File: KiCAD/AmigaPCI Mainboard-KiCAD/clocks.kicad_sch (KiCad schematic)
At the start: 30 parts, among them CN201 I2C, U108 74AHCT04, U201 Si5351A-B-GM, U210 AT27C4096, U211 AT27C4096, U219 74HCT04, U906 AT27C1024, U907 AT27C1024, Y3 25MHz

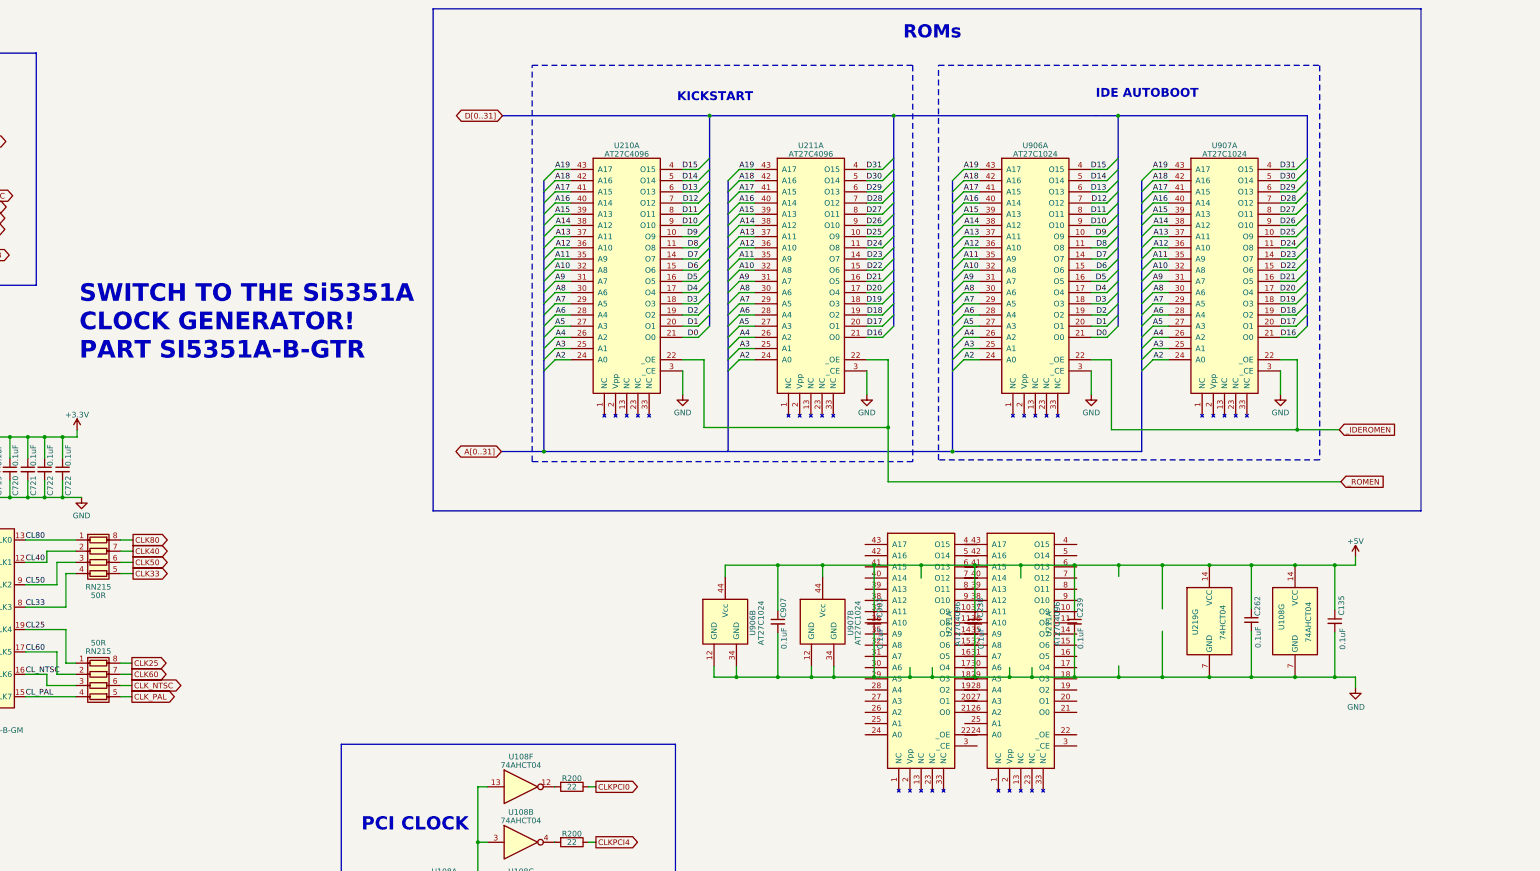
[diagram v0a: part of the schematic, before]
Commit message: Schematic and Routing 14-DEC-2023
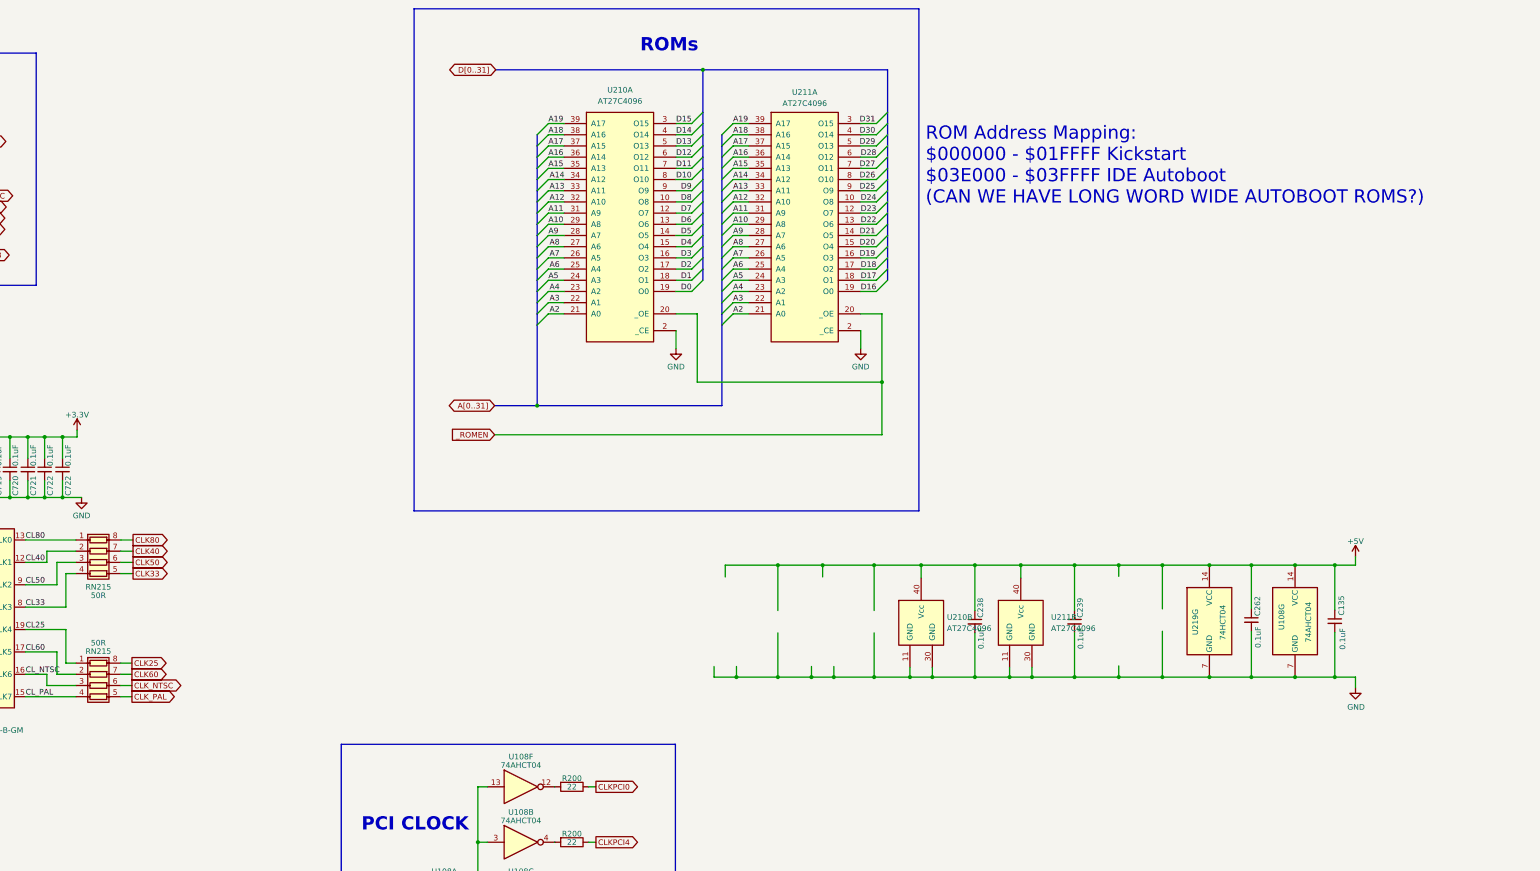
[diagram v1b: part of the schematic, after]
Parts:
- removed C903, C907: 0.1uF, Capacitor_SMD:C_0603_1608Metric, symbol Device:C_Small
- removed U210, U211 (x3): AT27C4096, Package_LCC:PLCC-44_SMD-Socket, symbol AmigaPCI-Symbols:AT27C4096-PLCC
- removed U906, U907: AT27C1024, Package_LCC:PLCC-44_SMD-Socket, symbol AmigaPCI-Symbols:AT27C4096-PLCC
- added U210, U211: AT27C4096, Package_DIP:DIP-40_W16.51mm_SMDSocket_LongPads, symbol AmigaPCI-Symbols:AT27C4096
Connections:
- net +5V: now also U210.40 (Vcc), U211.40 (Vcc)
- net A10: now also U210.29 (A8), U211.29 (A8)
- net A11: now also U210.31 (A9), U211.31 (A9)
- net A12: now also U210.32 (A10), U211.32 (A10)
- net A13: now also U210.33 (A11), U211.33 (A11)
- net A14: now also U210.34 (A12), U211.34 (A12)
- net A15: now also U210.35 (A13), U211.35 (A13)
- net A16: now also U210.36 (A14), U211.36 (A14)
- net A17: now also U210.37 (A15), U211.37 (A15)
- net A18: now also U210.38 (A16), U211.38 (A16)
- net A19: now also U210.39 (A17), U211.39 (A17)
- net A2: now also U210.21 (A0), U211.21 (A0)
- net A3: now also U210.22 (A1), U211.22 (A1)
- net A4: now also U210.23 (A2), U211.23 (A2)
- net A5: now also U210.24 (A3), U211.24 (A3)
- net A6: now also U210.25 (A4), U211.25 (A4)
- net A7: now also U210.26 (A5), U211.26 (A5)
- net A8: now also U210.27 (A6), U211.27 (A6)
- net A9: now also U210.28 (A7), U211.28 (A7)
- net D0: now also U210.19 (O0)
- net D1: now also U210.18 (O1)
- net D10: now also U210.8 (O10)
- net D11: now also U210.7 (O11)
- net D12: now also U210.6 (O12)
- net D13: now also U210.5 (O13)
- net D14: now also U210.4 (O14)
- net D15: now also U210.3 (O15)
- net D16: now also U211.19 (O0)
- net D17: now also U211.18 (O1)
- net D18: now also U211.17 (O2)
- net D19: now also U211.16 (O3)
- net D2: now also U210.17 (O2)
- net D20: now also U211.15 (O4)
- net D21: now also U211.14 (O5)
- net D22: now also U211.13 (O6)
- net D23: now also U211.12 (O7)
- net D24: now also U211.10 (O8)
- net D25: now also U211.9 (O9)
- net D26: now also U211.8 (O10)
- net D27: now also U211.7 (O11)
- net D28: now also U211.6 (O12)
- net D29: now also U211.5 (O13)
- net D3: now also U210.16 (O3)
- net D30: now also U211.4 (O14)
- net D31: now also U211.3 (O15)
- net D4: now also U210.15 (O4)
- net D5: now also U210.14 (O5)
- net D6: now also U210.13 (O6)
- net D7: now also U210.12 (O7)
- net D8: now also U210.10 (O8)
- net D9: now also U210.9 (O9)
- net GND: now also U210.11 (GND), U210.2 (_CE), U210.30 (GND), U211.11 (GND), U211.2 (_CE), U211.30 (GND)
- net _ROMEN: now also U210.20 (_OE), U211.20 (_OE)
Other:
- note added: "ROM Address Mapping: $000000 - $01FFFF Kickstart $03E000 - $03FFFF IDE Autoboot (CAN WE HAVE LONG WORD WIDE AUTOBOOT ROMS?)"
- note removed: "IDE AUTOBOOT"
- note removed: "KICKSTART"
- note removed: "SWITCH TO THE Si5351A CLOCK GENERATOR! PART SI5351A-B-GTR"

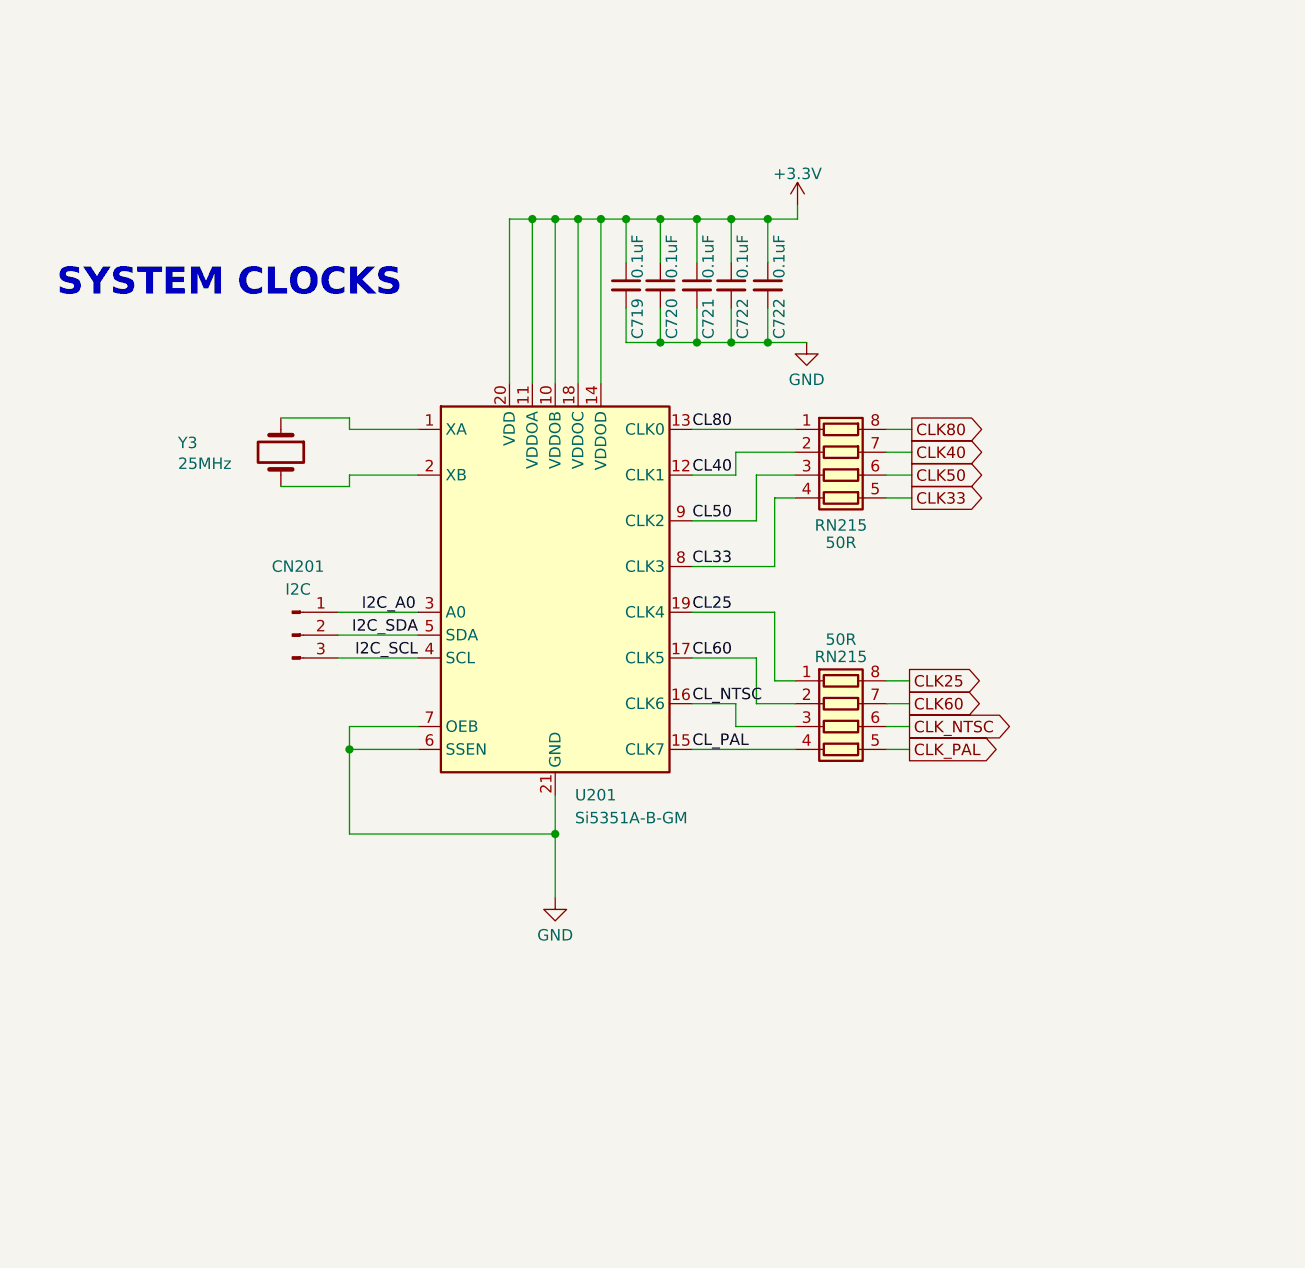
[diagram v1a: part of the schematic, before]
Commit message: Schematic Cleanup 15-DEC-2023
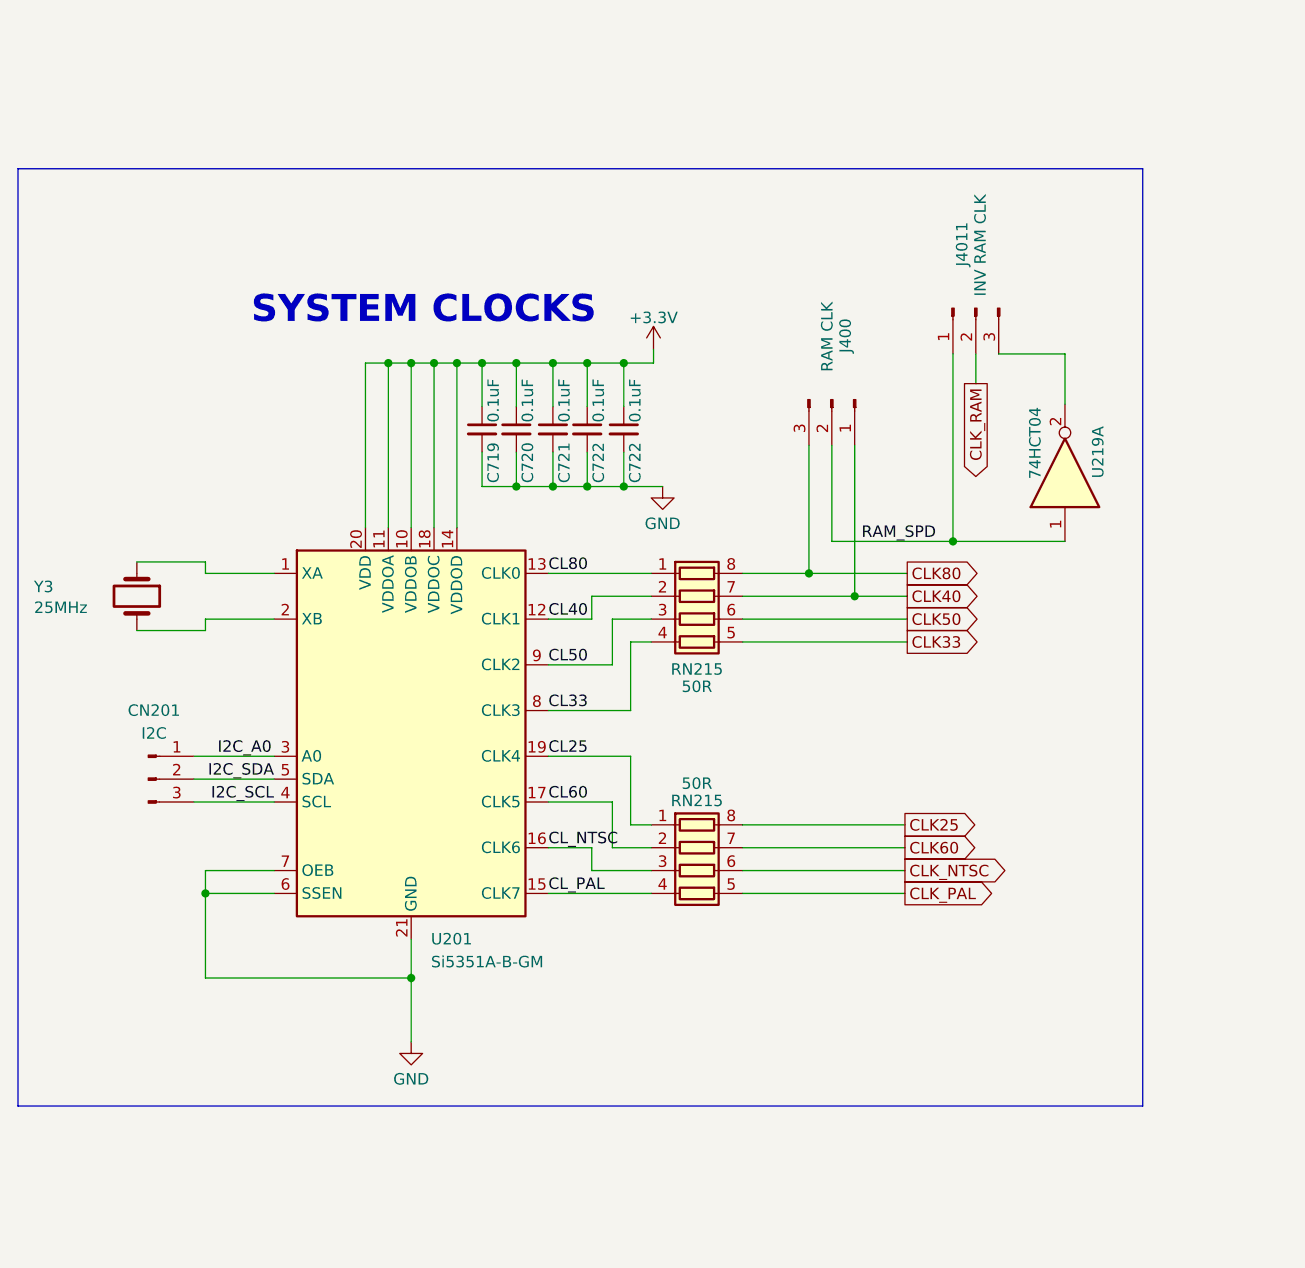
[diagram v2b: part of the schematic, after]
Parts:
- added J400: RAM CLK, Connector_PinHeader_2.54mm:PinHeader_1x03_P2.54mm_Vertical, symbol Connector:Conn_01x03_Pin
- added J4011: INV RAM CLK, Connector_PinHeader_2.54mm:PinHeader_1x03_P2.54mm_Vertical, symbol Connector:Conn_01x03_Pin
- added unit 1 of U219
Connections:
- net CLK40: now also J400.1 (Pin_1)
- net CLK80: now also J400.3 (Pin_3)
- new net: J4011.3 (Pin_3), U219.2
- new net CLK_RAM: J4011.2 (Pin_2)
- new net RAM_SPD: J400.2 (Pin_2), J4011.1 (Pin_1), U219.1
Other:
- moved on the sheet: C719, C720, C721, C722, CN201, RN215, U201, Y3
